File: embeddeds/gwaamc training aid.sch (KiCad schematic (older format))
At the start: 19 parts, among them J1 Conn_Coaxial, U1 LM334Z, U2 LM334Z, U3-A , U3-B U3_AD8244ARMZ, U3-C U3_AD8244ARMZ, U3-D U3_AD8244ARMZ, U4 74LV138 only needed with larg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, U5... 74LV138 only for large number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

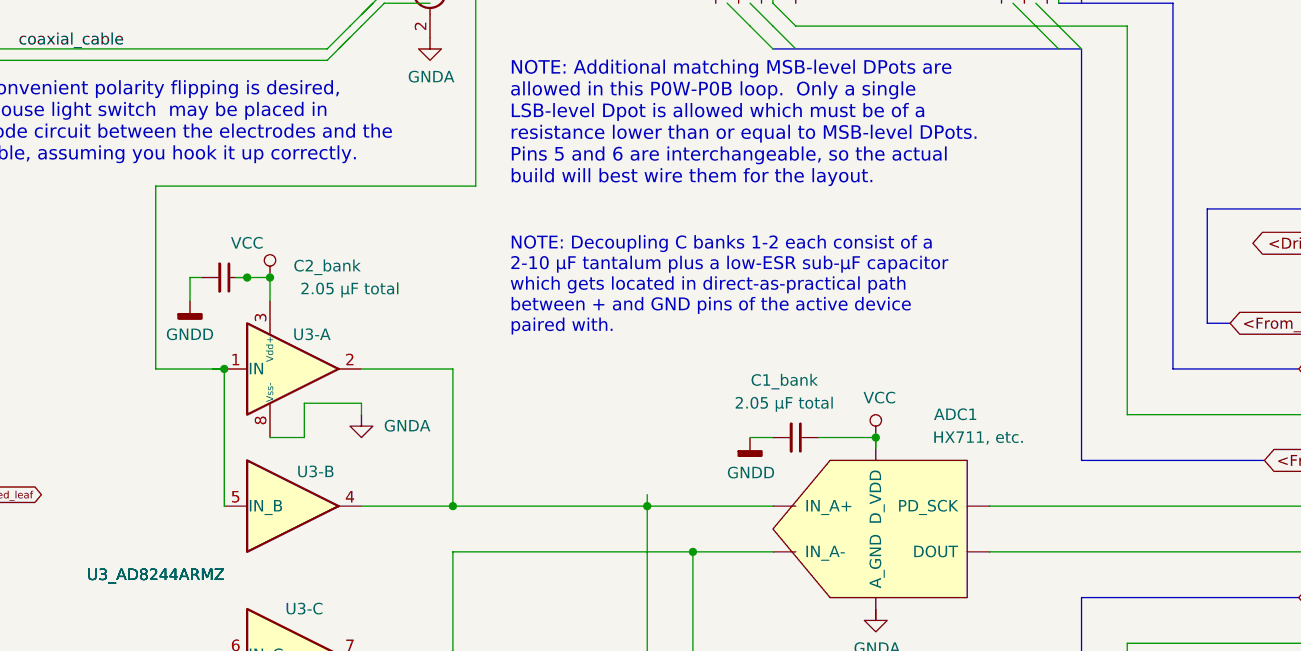
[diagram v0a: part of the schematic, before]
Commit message: Add files via upload
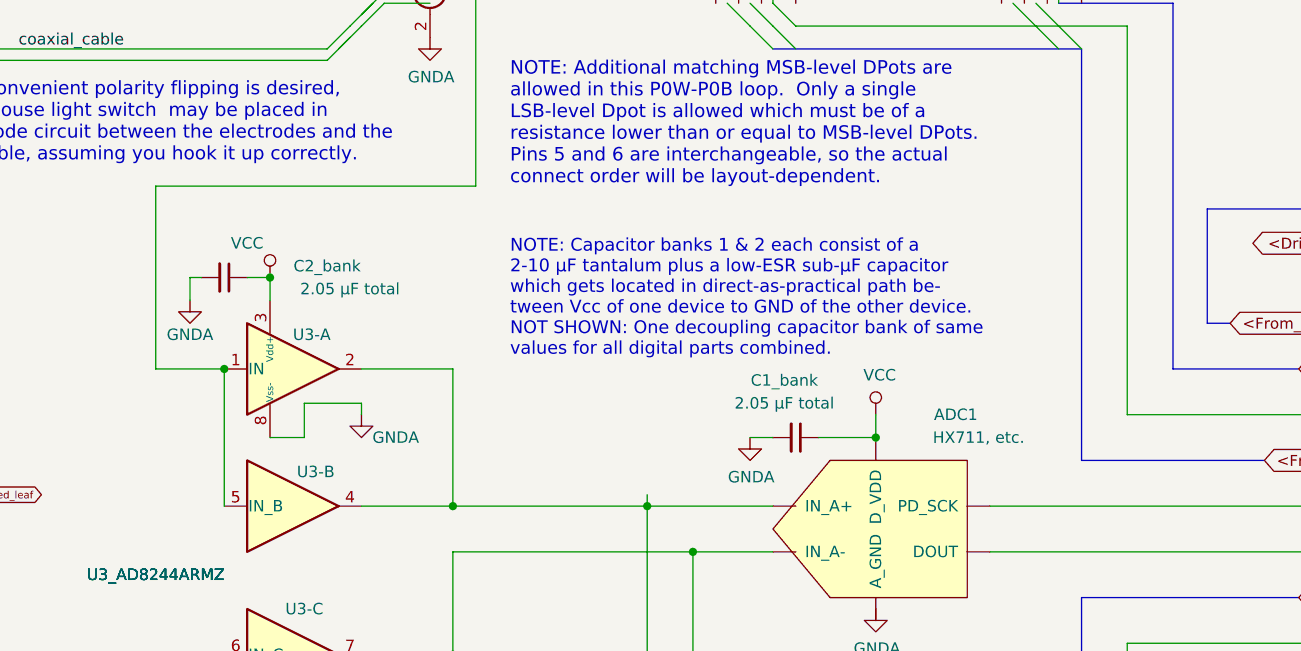
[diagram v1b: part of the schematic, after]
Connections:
- wire segments 92 -> 90
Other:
- note added: "NOTE: Additional matching MSB-level DPots are\nallowed in this P0W-P0B loop. Only a single \nLSB-level Dpot is allowed which must be of a\nresistance lower than or equal to MSB-level DPots.\nPins 5 and 6 are interchangeable, so the actual\nconnect order will be layout-dependent."
- note added: "NOTE: Capacitor banks 1 & 2 each consist of a \n2-10 µF tantalum plus a low-ESR sub-µF capacitor \nwhich gets located in direct-as-practical path be-\ntween Vcc of one device to GND of the other device. \nNOT SHOWN: One decoupling capacitor bank of same \nvalues for all digital parts combined."
- note removed: "NOTE: Additional matching MSB-level DPots are\nallowed in this P0W-P0B loop. Only a single \nLSB-level Dpot is allowed which must be of a\nresistance lower than or equal to MSB-level DPots.\nPins 5 and 6 are interchangeable, so the actual\nbuild will best wire them for the layout."
- note removed: "NOTE: Decoupling C banks 1-2 each consist of a \n2-10 µF tantalum plus a low-ESR sub-µF capacitor \nwhich gets located in direct-as-practical path \nbetween + and GND pins of the active device \npaired with."
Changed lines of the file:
@@
 <From_MCU_Digital_Pin_driving_this_CS
 Text Notes 3650 3200 0    59   ~ 0
-NOTE: Additional matching MSB-level DPots are\nallowed in this P0W-P0B loop.  Only a single \nLSB-level Dpot is allowed which must be of a\nresistance lower than or equal to MSB-level DPots.\nPins 5 and 6 are interchangeable, so the actual\nbuild will best wire them for the layout.
+NOTE: Additional matching MSB-level DPots are\nallowed in this P0W-P0B loop.  Only a single \nLSB-level Dpot is allowed which must be of a\nresistance lower than or equal to MSB-level DPots.\nPins 5 and 6 are interchangeable, so the actual\nconnect order will be layout-dependent.
 Text Notes 1000 3100 0    59   ~ 0
 NOTE: If convenient polarity flipping is desired,\n a 4-way house light switch  may be placed in \nthe electrode circuit between the electrodes and the \ncoaxial cable, assuming you hook it up correctly.
@@
 L power:GNDA #PWR?
 U 1 1 5C193F33
-P 3000 4200
-F 0 "#PWR?" H 3000 3950 50  0001 C CNN
-F 1 "GNDA" H 3200 4150 50  0000 C CNN
-F 2 "" H 3000 4200 50  0001 C CNN
-F 3 "" H 3000 4200 50  0001 C CNN
-	1    3000 4200
+P 2250 3700
+F 0 "#PWR?" H 2250 3450 50  0001 C CNN
+F 1 "GNDA" H 2250 3550 50  0000 C CNN
+F 2 "" H 2250 3700 50  0001 C CNN
+F 3 "" H 2250 3700 50  0001 C CNN
+	1    2250 3700
 	1    0    0    -1
 $EndComp
@@
 L power:VCC #PWR?
 U 1 1 5C19D6AB
-P 5250 4300
-F 0 "#PWR?" H 5250 4150 50  0001 C CNN
-F 1 "VCC" H 5267 4473 50  0000 C CNN
-F 2 "" H 5250 4300 50  0001 C CNN
-F 3 "" H 5250 4300 50  0001 C CNN
-	1    5250 4300
+P 5250 4200
+F 0 "#PWR?" H 5250 4050 50  0001 C CNN
+F 1 "VCC" H 5267 4373 50  0000 C CNN
+F 2 "" H 5250 4200 50  0001 C CNN
+F 3 "" H 5250 4200 50  0001 C CNN
+	1    5250 4200
 	1    0    0    -1
 $EndComp
@@
 $EndComp
 $Comp
-L power:GNDD #PWR?
-U 1 1 5C1C4E62
-P 4700 4300
-F 0 "#PWR?" H 4700 4050 50  0001 C CNN
-F 1 "GNDD" H 4704 4145 50  0000 C CNN
-F 2 "" H 4700 4300 50  0001 C CNN
-F 3 "" H 4700 4300 50  0001 C CNN
-	1    4700 4300
-	1    0    0    -1
-$EndComp
-$Comp
 L Device:C_Small C2_bank
 U 1 1 5C1C5AE4
@@
 	0    1    1    0
 $EndComp
-$Comp
-L power:GNDD #PWR?
-U 1 1 5C1C6E06
-P 2250 3700
-F 0 "#PWR?" H 2250 3450 50  0001 C CNN
-F 1 "GNDD" H 2250 3550 50  0000 C CNN
-F 2 "" H 2250 3700 50  0001 C CNN
-F 3 "" H 2250 3700 50  0001 C CNN
-	1    2250 3700
-	1    0    0    -1
-$EndComp
 Wire Wire Line
 	10350 4450 10500 4450
@@
 Text Notes 9150 6450 0    56   ~ 0
 *NOTE FOR MCU ANALOG PINS:  Low-\nnumbered Analog Input pins are reserved \nfor all existing DPOT-controlled leg outputs.  \nUnused Analog Pins above them may be\nused to display additional plotter traces\nwhen so defined in preprocessor macros.
-Text Notes 3650 3850 0    56   ~ 0
-NOTE: Decoupling C banks 1-2 each consist of a \n2-10 µF tantalum plus a low-ESR sub-µF capacitor \nwhich gets located in direct-as-practical path \nbetween + and GND pins of the active device \npaired with.
+Text Notes 3650 3950 0    56   ~ 0
+NOTE: Capacitor banks 1 & 2 each consist of a \n2-10 µF tantalum plus a low-ESR sub-µF capacitor \nwhich gets located in direct-as-practical path be-\ntween Vcc of one device to GND of the other device.  \nNOT SHOWN: One decoupling capacitor bank of same \nvalues for all digital parts combined.
 Text Notes 650  1300 0    66   ~ 0
 NOTE:  The LM334 devices must receive 5 VDC or greater due to their own operating voltage range.  \nTheir functional range will be substantially limited if powered by the 3 or 3.3 VDC of many MCUs.  \nProvide a dedicated positive power supply to them if 5 VDC is not otherwise available, then carefully \nensure the output levels from them are prevented from exceeding the input range of the remaining \ncircuitry.
@@
 Wire Wire Line
 	4800 4300 4700 4300
-Wire Wire Line
-	5250 4300 5250 4350
-Connection ~ 5250 4300
-Wire Wire Line
-	5000 4300 5250 4300
 Connection ~ 2900 6900
 Entry Wire Line
@@
 	2900 6900 2900 7150
 Wire Wire Line
-	2450 3600 2500 3600
-Wire Wire Line
 	2900 1550 2900 2150
 Wire Wire Line
@@
 Wire Wire Line
 	6350 7050 6350 5200
-Connection ~ 2500 3600
-Wire Wire Line
-	2500 3600 2600 3600
 Connection ~ 4250 4600
 Wire Wire Line
 	4250 4600 4250 5600
-Wire Wire Line
-	2350 4000 2400 4000
 Wire Wire Line
 	2100 4000 2400 4000
@@
 1
 Wire Wire Line
+	2500 3600 2600 3600
+Wire Wire Line
+	5250 4200 5250 4300
+Wire Wire Line
+	5000 4300 5250 4300
+Connection ~ 5250 4300
+$Comp
+L power:GNDA #PWR?
+U 1 1 5C1E5690
+P 3000 4200
+F 0 "#PWR?" H 3000 3950 50  0001 C CNN
+F 1 "GNDA" H 3150 4100 50  0000 C CNN
+F 2 "" H 3000 4200 50  0001 C CNN
+F 3 "" H 3000 4200 50  0001 C CNN
+	1    3000 4200
+	1    0    0    -1
+$EndComp
+$Comp
+L power:GNDA #PWR?
+U 1 1 5C1E56EB
+P 4700 4300
+F 0 "#PWR?" H 4700 4050 50  0001 C CNN
+F 1 "GNDA" H 4705 4127 50  0000 C CNN
+F 2 "" H 4700 4300 50  0001 C CNN
+F 3 "" H 4700 4300 50  0001 C CNN
+	1    4700 4300
+	1    0    0    -1
+$EndComp
+Wire Wire Line
 	1300 5350 1300 7100
